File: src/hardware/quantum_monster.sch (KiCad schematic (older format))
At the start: 25 parts, among them J1 ICSP, J2 PCD8544, Q1 VS1838B, SW1 RESET, SW2 A, SW3 B, SW4 C, U1 ATmega328P-PU, Y1 32.768kHz

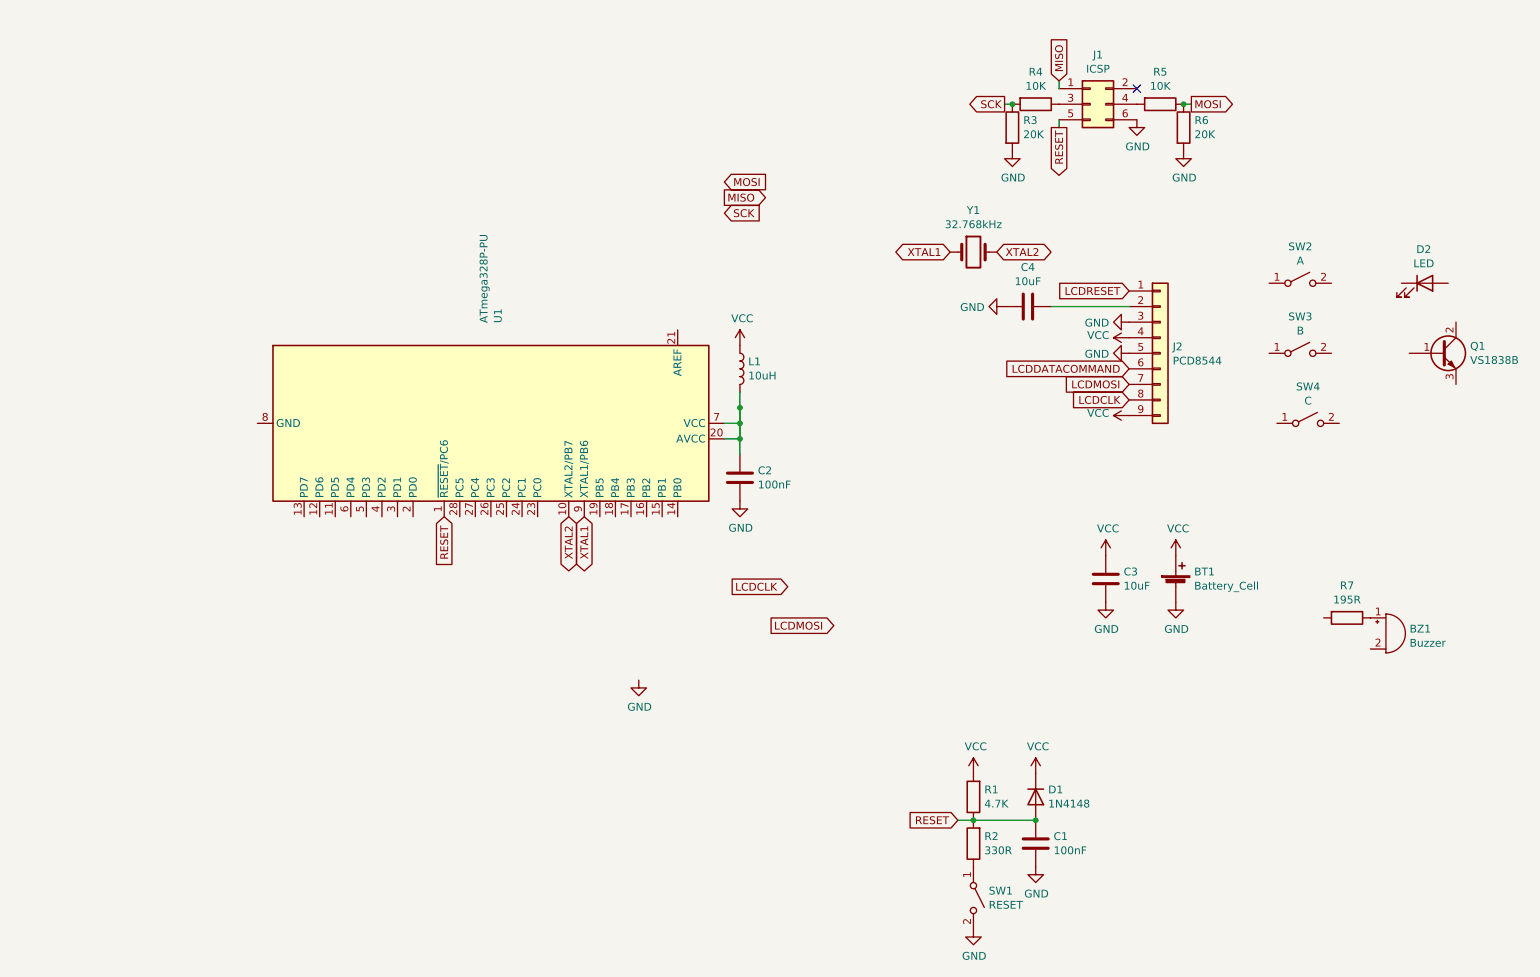
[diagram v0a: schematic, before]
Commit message: Continue experimenting with hardware design.
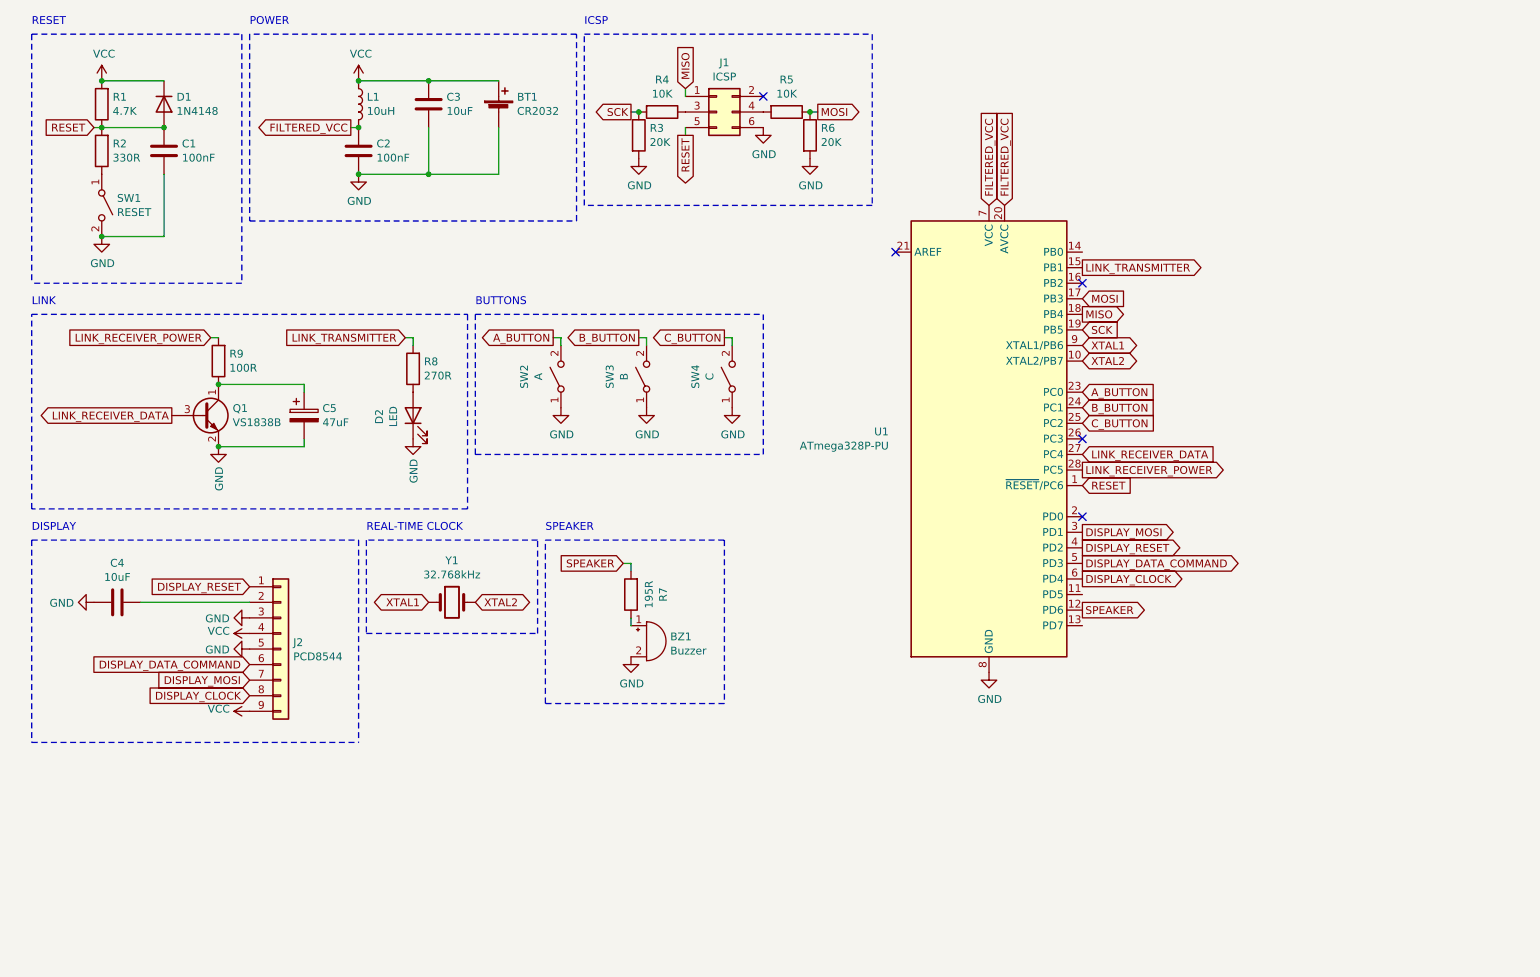
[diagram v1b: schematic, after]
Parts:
- removed Q1: VS1838B, Package_TO_SOT_THT:TO-92_Inline_Wide, symbol Device:Q_NPN_BCE
- added C5: 47uF, Capacitor_THT:CP_Radial_D5.0mm_P2.00mm, symbol Device:CP
- added Q1: VS1838B, Package_TO_SOT_THT:TO-92L_Inline_Wide, symbol Transistor_BJT:BC240
- added R8: 270R, Resistor_THT:R_Axial_DIN0204_L3.6mm_D1.6mm_P7.62mm_Horizontal, symbol Device:R
- added R9: 100R, Resistor_THT:R_Axial_DIN0204_L3.6mm_D1.6mm_P7.62mm_Horizontal, symbol Device:R
- BT1: value Battery_Cell -> CR2032
- C1, C2: footprint (none) -> Capacitor_THT:C_Disc_D5.0mm_W2.5mm_P2.50mm
- C3: footprint (none) -> Capacitor_THT:C_Disc_D4.3mm_W1.9mm_P5.00mm
- C4: footprint Capacitor_THT:C_Disc_D5.0mm_W2.5mm_P5.00mm -> Capacitor_THT:C_Disc_D4.3mm_W1.9mm_P5.00mm
- D2: footprint LED_THT:LED_D5.0mm -> LED_THT:LED_D5.0mm_IRBlack
- L1: footprint (none) -> Inductor_THT:L_Axial_L5.3mm_D2.2mm_P7.62mm_Horizontal_Vishay_IM-1
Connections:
- net LCDCLK is gone; now on net DISPLAY_CLOCK: J2.8 (Pin_8)
- net LCDDATACOMMAND is gone; now on net DISPLAY_DATA_COMMAND: J2.6 (Pin_6)
- net LCDMOSI is gone; now on net DISPLAY_MOSI: J2.7 (Pin_7)
- net LCDRESET is gone; now on net DISPLAY_RESET: J2.1 (Pin_1)
- net GND: now also BZ1.2 (+), D2.1 (K), SW2.1 (A), SW3.1 (A), SW4.1 (A), U1.22 (GND), U1.8 (GND), C5.2, Q1.2 (E)
- net MISO: now also U1.18 (PB4)
- net MOSI: now also U1.17 (PB3)
- net SCK: now also U1.19 (PB5)
- net SPEAKER: now reaches U1.12 (PD6)
- net SPEAKER: now also R7.2
- net LINK_TRANSMITTER: now reaches U1.15 (PB1)
- net LINK_TRANSMITTER: now also R8.2
- net FILTERED_VCC: now reaches C2.1, L1.2, U1.20 (AVCC), U1.7 (VCC)
- net A_BUTTON: now reaches U1.23 (PC0)
- net A_BUTTON: now also SW2.2 (B)
- net B_BUTTON: now reaches U1.24 (PC1)
- net B_BUTTON: now also SW3.2 (B)
- net C_BUTTON: now reaches U1.25 (PC2)
- net C_BUTTON: now also SW4.2 (B)
- net LINK_RECEIVER_DATA: now reaches U1.27 (PC4)
- net LINK_RECEIVER_DATA: now also Q1.3 (B)
- net LINK_RECEIVER_POWER: now reaches U1.28 (PC5)
- net LINK_RECEIVER_POWER: now also R9.2
- net DISPLAY_MOSI: now reaches U1.3 (PD1)
- net DISPLAY_RESET: now reaches U1.4 (PD2)
- net DISPLAY_DATA_COMMAND: now reaches U1.5 (PD3)
- net DISPLAY_CLOCK: now reaches U1.6 (PD4)
- net at D2.2 (A): now also R8.1
- new net: C5.1, Q1.1 (C), R9.1
- no-connect marks 1 -> 5
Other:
- note added: "BUTTONS"
- note added: "DISPLAY"
- note added: "ICSP"
- note added: "LINK"
- note added: "POWER"
- note added: "REAL-TIME CLOCK"
- note added: "RESET"
- note added: "SPEAKER"
- moved on the sheet: BT1, BZ1, C1, C2, C3, C4, D1, D2, J1, J2, L1, R1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
